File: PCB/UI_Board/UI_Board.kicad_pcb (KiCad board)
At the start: 2 copper layers, 169.8 x 35 mm, 18 parts, among them J1 DISPLAY, J2 CABLE, SW1 SW_UP, SW2 SW_DWN, SW3 SW_PRE_1, SW4 SW_PRE_2

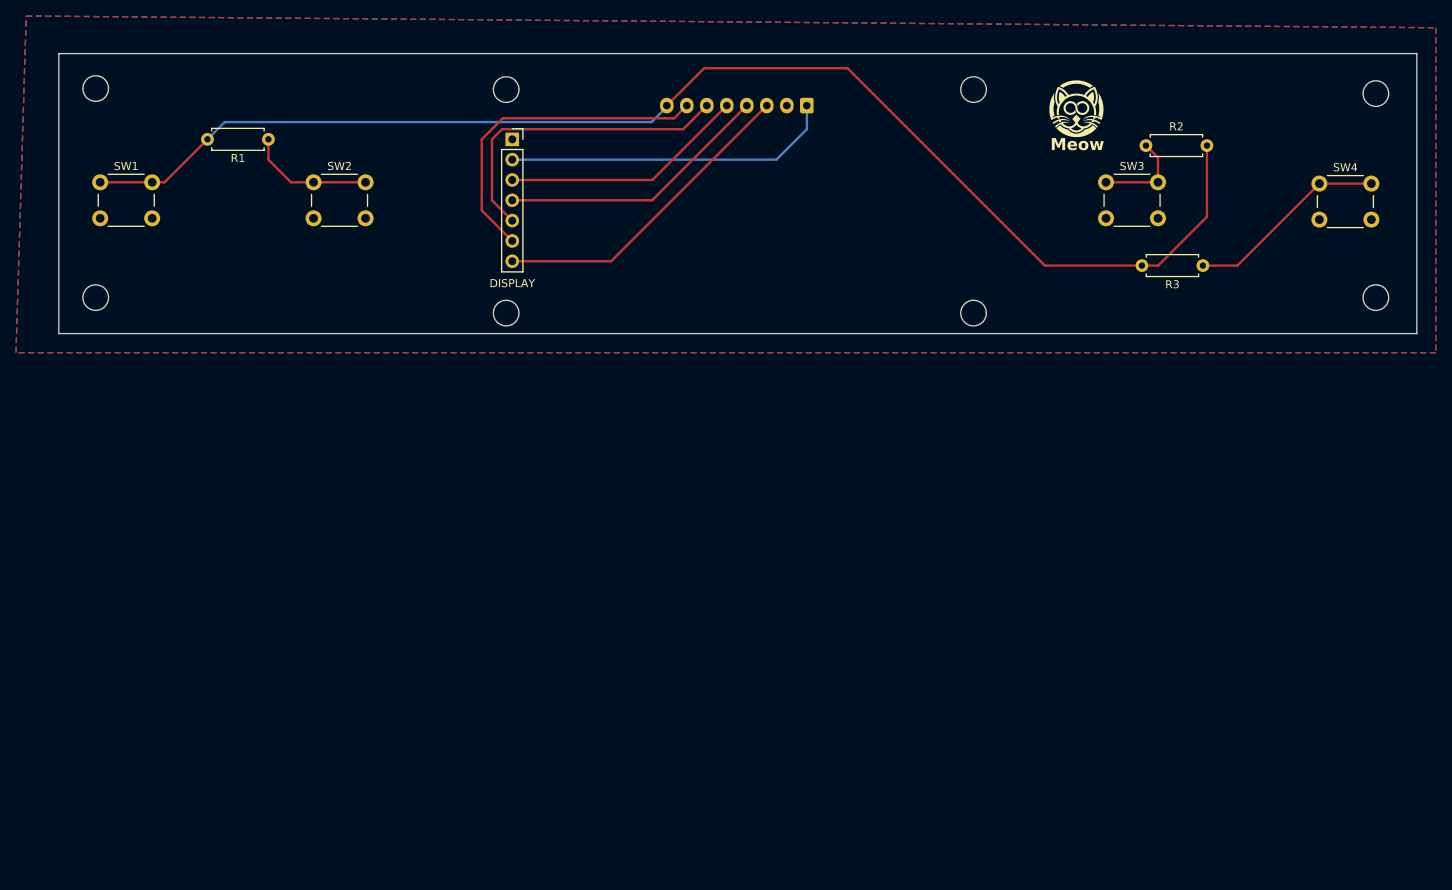
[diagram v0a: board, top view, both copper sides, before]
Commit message: Updated PCB files
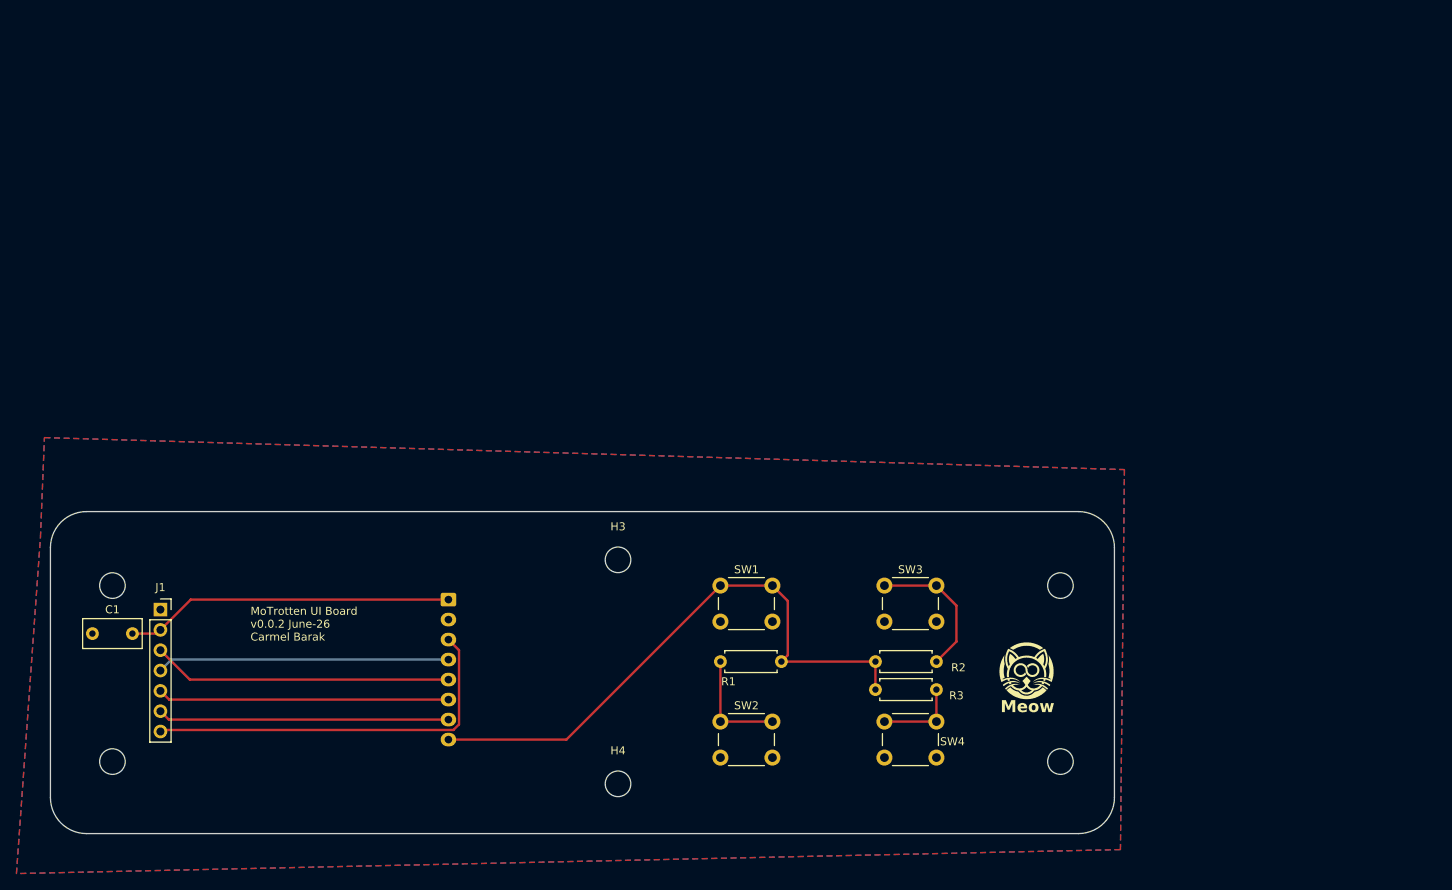
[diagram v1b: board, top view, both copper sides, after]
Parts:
- removed H1, H2: MountingHole, MountingHole:MountingHole_3.2mm_M3
- added C1: 0.1uF, Capacitor_THT:C_Rect_L7.2mm_W3.5mm_P5.00mm_FKS2_FKP2_MKS2_MKP2, F.Cu at (41.5, 107.5)
- moved H3 100.2 mm to (107.2, 98.3)
- moved H8 97.4 mm to (44.0, 123.5)
- moved SW1 92.5 mm to (120.0, 101.5)
- moved H4 89.2 mm to (107.2, 126.3)
- moved SW4 86.5 mm to (140.5, 118.5)
- moved R1 86.3 mm to (120.0, 111.0), turned to 0 degrees
- moved H5 84.7 mm to (162.5, 123.5)
- moved SW2 84.4 mm to (120.0, 118.5)
- moved J2 76.3 mm to (86.0, 103.2), turned to -90 degrees
- moved J1 73.4 mm to (50.0, 104.5)
- moved ? 70.5 mm to (161.1, 110.4)
- moved R2 69.6 mm to (147.0, 111.0), turned to 180 degrees
- moved R3 62.6 mm to (147.0, 114.5)
- moved H7 59.9 mm to (44.0, 101.5)
- moved SW3 57.5 mm to (140.5, 101.5)
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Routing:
- net /BTNS: track 167.5 -> 74.5 mm
- net Net-(R3-Pad1): track 25.3 -> 10.5 mm
- net /CS: track 39.9 -> 48.8 mm
- net /SCL: track 30.7 -> 37.5 mm
- net Net-(R2-Pad1): track 11.9 -> 18.1 mm
- net /DC: track 41.7 -> 36.4 mm
- net /RST: track 39.8 -> 36.5 mm
- net /SDA: track 34.2 -> 36.6 mm
- net Net-(R1-Pad1): track 15.9 -> 14.0 mm
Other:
- board size 169.8 x 35 mm -> 133 x 40.2 mm
- board text added: "DISPLAY"
- board text added: "MoTrotten UI Board v0.0.2 June-26 Carmel Barak"
